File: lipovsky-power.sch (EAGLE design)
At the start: 97 parts, among them J1 M04-929J, J2 M04-929J, J3 M04-929J, J4 M04-929J, Q1 NMOS30V_30A, Q12 NMOS40V_10A, Q14 NMOS40V_10A, Q16 NMOS40V_10A, Q18 NMOS40V_10A, Q21 PMOS30V_11A, Q22 PMOS30V_11A, Q23 NMOS40V_10A, Q24 NMOS40V_10A, Q25 PMOS30V_11A, Q26 PMOS30V_11A, Q27 NMOS40V_10A, Q28 NMOS40V_10A, Q3 2PMOS50V_0.17A, Q31 PMOS30V_11A, Q32 PMOS30V_11A, Q33 PMOS30V_11A, Q34 PMOS30V_11A, Q35 PMOS30V_11A, Q36 PMOS30V_11A, Q37 PMOS30V_11A, Q38 PMOS30V_11A, Q4 2PMOS50V_0.17A, Q41 PMOS30V_11A, Q42 PMOS30V_11A, Q43 PMOS30V_11A, Q44 PMOS30V_11A, Q45 PMOS30V_11A, Q46 PMOS30V_11A, Q47 PMOS30V_11A, Q48 PMOS30V_11A, Q5 2NMOS30V_0.1A, Q51 PMOS30V_11A, Q52 PMOS30V_11A, Q53 PMOS30V_11A, Q54 PMOS30V_11A, Q55 PMOS30V_11A, Q56 PMOS30V_11A, Q57 PMOS30V_11A, Q58 PMOS30V_11A, Q62 PMOS30V_11A, Q64 PMOS30V_11A, Q66 PMOS30V_11A, Q68 PMOS30V_11A, T1 TFORM_4_4311_4A4, U1 DG508BEN-T1-GE4, U2 DG508BEN-T1-GE4, U4 LTC3805-5IDD, U6 AR30N60PPA-13

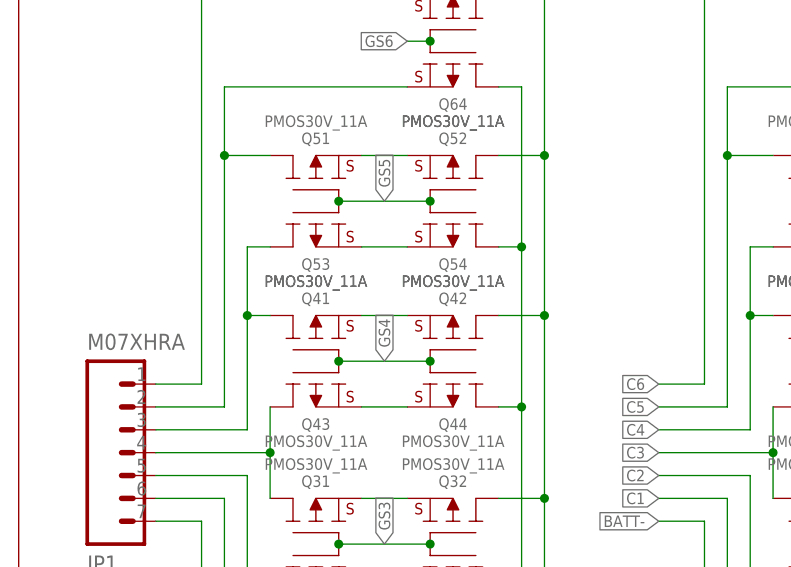
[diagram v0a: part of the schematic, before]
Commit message: test point
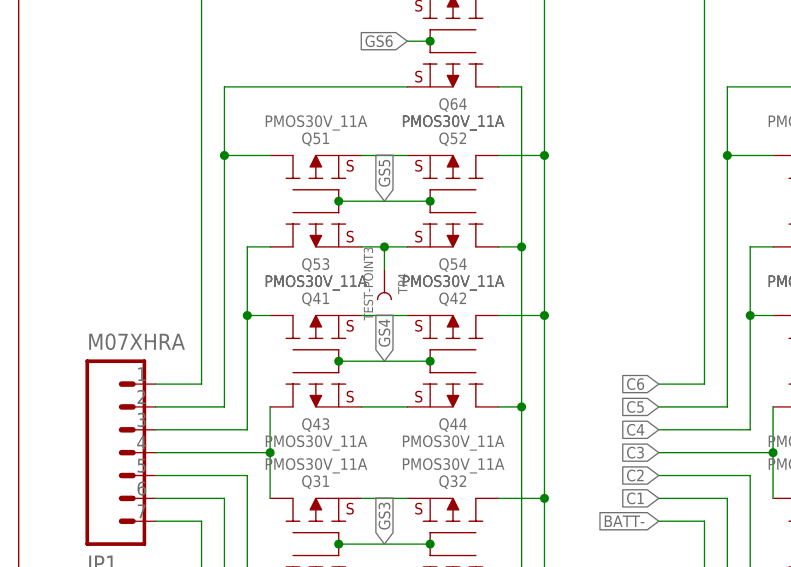
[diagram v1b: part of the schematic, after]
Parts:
- added TP4: TEST-POINT3, SparkFun-Passives:TEST-POINT3
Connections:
- net SS-5: now also TP4.1
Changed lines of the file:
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@@
 <part name="R10" library="dubec" deviceset="RES" device="10K_16"/>
 <part name="R19" library="dubec" deviceset="RES" device="10K_16"/>
+<part name="TP4" library="SparkFun-Passives" deviceset="TEST-POINT" device="3"/>
 </parts>
 <sheets>
@@
 <instance part="R10" gate="G$1" x="114.3" y="22.86"/>
 <instance part="R19" gate="G$1" x="200.66" y="22.86"/>
+<instance part="TP4" gate="G$1" x="-93.98" y="20.32" rot="R270"/>
 </instances>
 <busses>
@@
 <net name="SS+5" class="0">
 <segment>
-<wire x1="-96.52" y1="33.02" x2="-91.44" y2="33.02" width="0.1524" layer="91"/>
 <pinref part="Q51" gate="G$1" pin="S"/>
 <pinref part="Q52" gate="G$1" pin="S"/>
+<wire x1="-96.52" y1="33.02" x2="-91.44" y2="33.02" width="0.1524" layer="91"/>
 </segment>
 </net>
 <net name="SS-5" class="0">
 <segment>
-<wire x1="-91.44" y1="22.86" x2="-96.52" y2="22.86" width="0.1524" layer="91"/>
+<wire x1="-91.44" y1="22.86" x2="-93.98" y2="22.86" width="0.1524" layer="91"/>
 <pinref part="Q54" gate="G$1" pin="S"/>
 <pinref part="Q53" gate="G$1" pin="S"/>
-</segment>
-</net>
+<pinref part="TP4" gate="G$1" pin="1"/>
+<wire x1="-93.98" y1="22.86" x2="-96.52" y2="22.86" width="0.1524" layer="91"/>
+<wire x1="-93.98" y1="20.32" x2="-93.98" y2="22.86" width="0.1524" layer="91"/>
+<junction x="-93.98" y="22.86"/>
+</segment>
+</net>
